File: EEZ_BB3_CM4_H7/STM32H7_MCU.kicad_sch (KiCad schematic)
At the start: 64 parts, among them IC2 STM32H757IIT6, IC3 AP1117-33, Y1 XTAL016178-85SMX

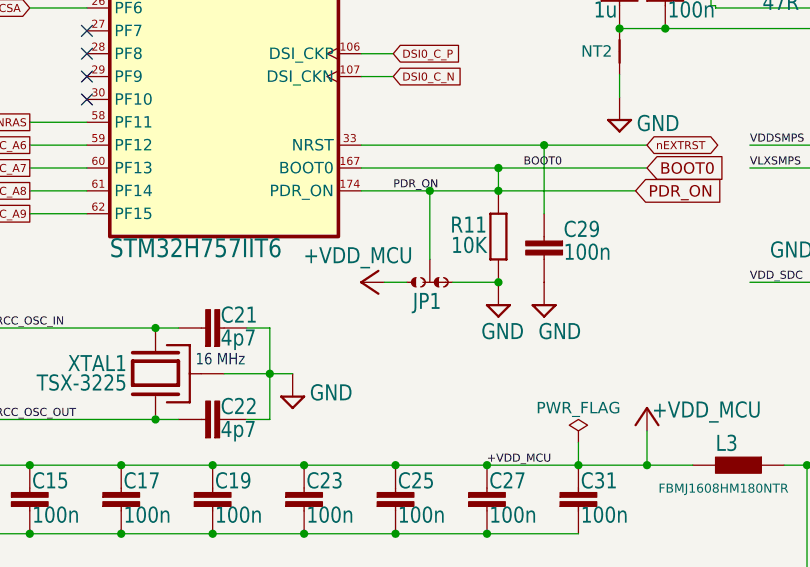
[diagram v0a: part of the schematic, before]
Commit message: Fixing errors - adding README
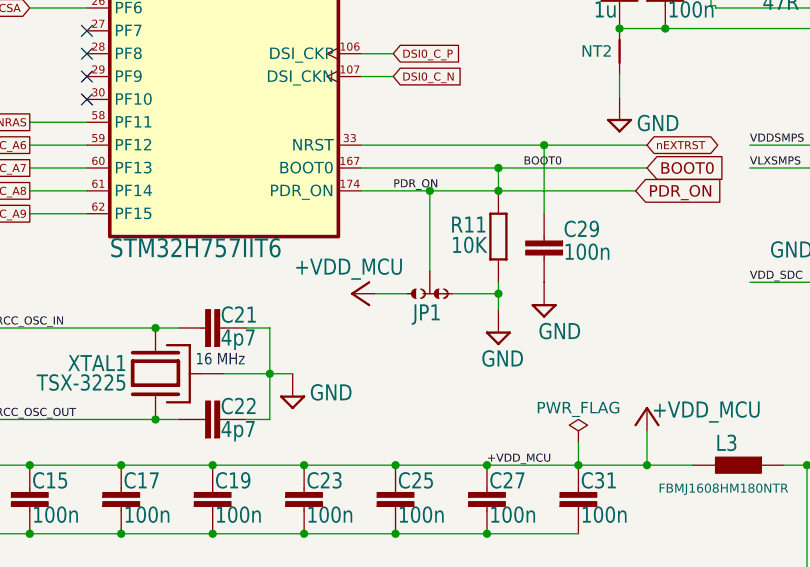
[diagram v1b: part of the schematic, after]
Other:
- moved on the sheet: JP1
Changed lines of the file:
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@@
   (junction (at 130.81 134.62) (diameter 0) (color 0 0 0 0)
   )
-  (junction (at 193.04 114.3) (diameter 0) (color 0 0 0 0)
+  (junction (at 193.04 115.57) (diameter 0) (color 0 0 0 0)
   )
   (junction (at 233.68 67.31) (diameter 0) (color 0 0 0 0)
@@
     (stroke (width 0.1524) (type solid))
   )
+  (wire (pts (xy 193.04 117.348) (xy 193.04 115.57))
+    (stroke (width 0) (type default))
+  )
   (wire (pts (xy 233.68 104.14) (xy 233.68 95.25))
     (stroke (width 0.1524) (type solid))
@@
     (stroke (width 0.1524) (type solid))
   )
+  (wire (pts (xy 187.96 115.57) (xy 193.04 115.57))
+    (stroke (width 0.1524) (type solid))
+  )
   (wire (pts (xy 266.7 55.88) (xy 269.24 55.88))
     (stroke (width 0.1524) (type solid))
@@
     (stroke (width 0.1524) (type solid))
   )
+  (wire (pts (xy 179.324 115.57) (xy 182.88 115.57))
+    (stroke (width 0.1524) (type solid))
+  )
   (wire (pts (xy 140.97 154.94) (xy 130.81 154.94))
     (stroke (width 0.1524) (type solid))
@@
     (stroke (width 0.1524) (type solid))
   )
-  (wire (pts (xy 182.88 114.3) (xy 180.34 114.3))
-    (stroke (width 0.1524) (type solid))
-  )
   (wire (pts (xy 140.97 134.62) (xy 130.81 134.62))
     (stroke (width 0.1524) (type solid))
@@
     (stroke (width 0.1524) (type solid))
   )
+  (wire (pts (xy 193.04 115.57) (xy 193.04 114.3))
+    (stroke (width 0) (type default))
+  )
   (wire (pts (xy 233.68 43.18) (xy 233.68 45.72))
     (stroke (width 0.1524) (type solid))
@@
     (stroke (width 0.1524) (type solid))
   )
-  (wire (pts (xy 187.96 114.3) (xy 193.04 114.3))
-    (stroke (width 0.1524) (type solid))
-  )
   (wire (pts (xy 229.362 73.406) (xy 229.362 81.026))
     (stroke (width 0.1524) (type solid))
@@
     (stroke (width 0) (type default))
   )
-  (wire (pts (xy 185.42 111.76) (xy 185.42 104.14))
+  (wire (pts (xy 185.42 113.03) (xy 185.42 104.14))
     (stroke (width 0.1524) (type solid))
   )
@@
     )
   )
-  (symbol (lib_id "Envox H745 Master MCU r2B6-eagle-import:GND") (at 193.04 116.84 0) (mirror y) (unit 1)
+  (symbol (lib_id "Envox H745 Master MCU r2B6-eagle-import:GND") (at 193.04 119.888 0) (mirror y) (unit 1)
     (in_bom yes) (on_board yes) (dnp no)
-    (property "Reference" "#SUPPLY012" (at 193.04 116.84 0)
+    (property "Reference" "#SUPPLY012" (at 193.04 119.888 0)
       (effects (font (size 1.27 1.27)) hide)
     )
-    (property "Value" "GND" (at 191.135 118.745 0)
+    (property "Value" "GND" (at 191.135 121.793 0)
       (effects (font (size 1.778 1.5113)) (justify right top))
     )
-    (property "Footprint" "" (at 193.04 116.84 0)
+    (property "Footprint" "" (at 193.04 119.888 0)
       (effects (font (size 1.27 1.27)) hide)
     )
-    (property "Datasheet" "" (at 193.04 116.84 0)
+    (property "Datasheet" "" (at 193.04 119.888 0)
       (effects (font (size 1.27 1.27)) hide)
     )
@@
     )
   )
-  (symbol (lib_id "Envox H745 Master MCU r2B6-eagle-import:+VDD_MCU") (at 180.34 114.3 90) (mirror x) (unit 1)
+  (symbol (lib_id "Envox H745 Master MCU r2B6-eagle-import:+VDD_MCU") (at 179.324 115.57 90) (mirror x) (unit 1)
     (in_bom yes) (on_board yes) (dnp no)
-    (property "Reference" "#+VDD_MCU01" (at 180.34 114.3 0)
+    (property "Reference" "#+VDD_MCU01" (at 179.324 115.57 0)
       (effects (font (size 1.27 1.27)) hide)
     )
-    (property "Value" "+VDD_MCU" (at 183.515 112.395 90)
+    (property "Value" "+VDD_MCU" (at 182.499 113.665 90)
       (effects (font (size 1.778 1.5113)) (justify left bottom))
     )
-    (property "Footprint" "" (at 180.34 114.3 0)
+    (property "Footprint" "" (at 179.324 115.57 0)
       (effects (font (size 1.27 1.27)) hide)
     )
-    (property "Datasheet" "" (at 180.34 114.3 0)
+    (property "Datasheet" "" (at 179.324 115.57 0)
       (effects (font (size 1.27 1.27)) hide)
     )
@@
     )
   )
-  (symbol (lib_id "Library:JP3-CUT-0805-ROTATED") (at 185.42 114.3 90) (unit 1)
+  (symbol (lib_id "Library:JP3-CUT-0805-ROTATED") (at 185.42 115.57 90) (unit 1)
     (in_bom no) (on_board yes) (dnp no)
-    (property "Reference" "JP1" (at 183.515 117.475 90)
+    (property "Reference" "JP1" (at 183.515 118.745 90)
       (effects (font (size 1.778 1.5113)) (justify right top))
     )
-    (property "Value" "JP3-CUT-0805-ROTATED" (at 185.42 114.3 0)
+    (property "Value" "JP3-CUT-0805-ROTATED" (at 185.42 115.57 0)
       (effects (font (size 1.27 1.27)) hide)
     )
-    (property "Footprint" "Library:JP3-0805-CUT2" (at 185.42 114.3 0)
+    (property "Footprint" "Library:JP3-0805-CUT2" (at 185.42 115.57 0)
       (effects (font (size 1.27 1.27)) hide)
     )
-    (property "Datasheet" "" (at 185.42 114.3 0)
+    (property "Datasheet" "" (at 185.42 115.57 0)
       (effects (font (size 1.27 1.27)) hide)
     )
